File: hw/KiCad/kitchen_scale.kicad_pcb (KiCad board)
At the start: 2 copper layers, 59 x 50 mm, 11 parts, among them J1 Conn_01x08_Socket, J2 Conn_HX711, SW1 SW_Push, SW2 SW_SPST, SW3 SW_Push, SW4 SW_Push, U1 DEBO1_3_7LI_1_0A charge_contr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, U2 WeMos_D1_mini, U3 LF33_TO220

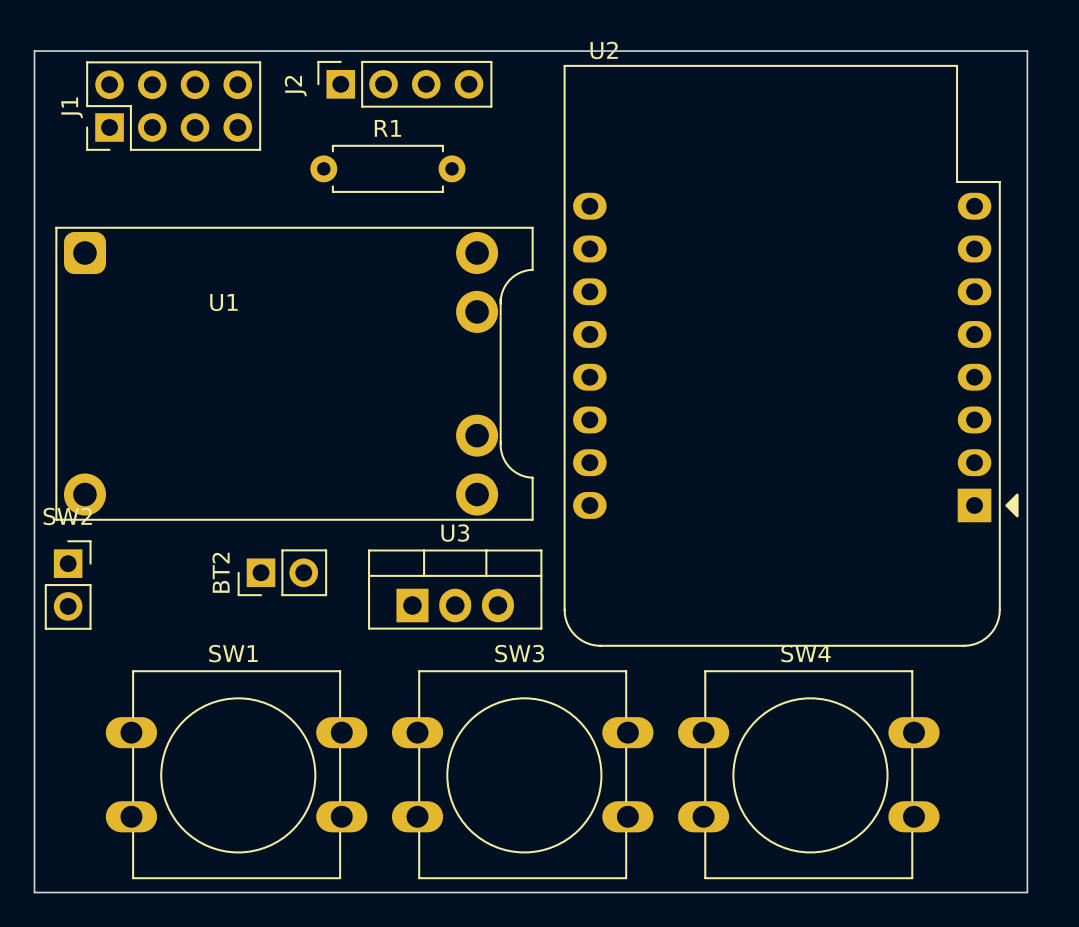
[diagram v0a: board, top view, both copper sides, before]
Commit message: Update of fine placement
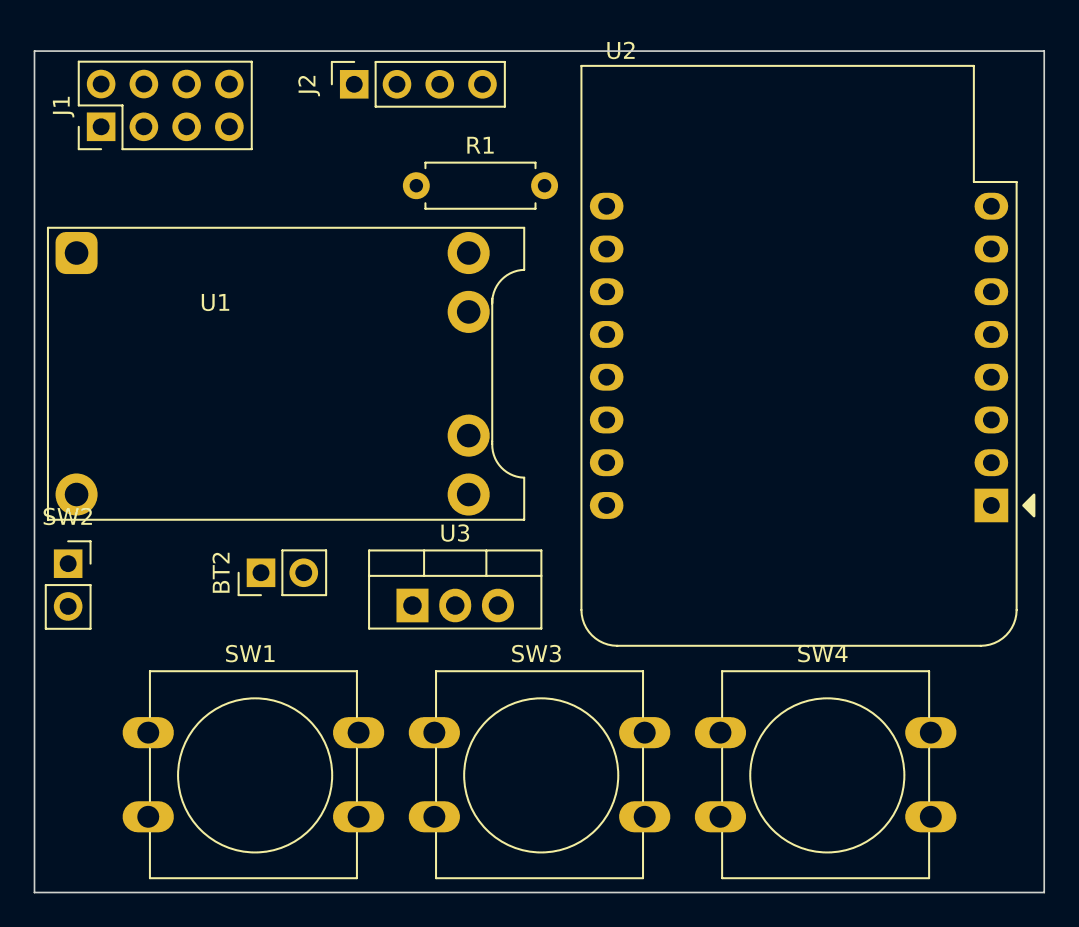
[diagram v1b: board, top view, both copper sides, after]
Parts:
- moved R1 5.59 mm to (82.7, 83.0)
- moved SW1 1.00 mm to (66.8, 115.5)
- moved SW3 1.00 mm to (83.8, 115.5)
- moved SW4 1.00 mm to (100.8, 115.5)
- moved U2 1.00 mm to (116.9, 102.0)
- moved J2 0.80 mm to (79.0, 77.0)
- moved J1 0.50 mm to (64.0, 79.5)
- moved U1 0.50 mm to (60.8, 92.5)
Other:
- board size 59 x 50 mm -> 60 x 50 mm
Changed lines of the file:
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@@
   (net 22 "unconnected-(U2-TX-Pad16)")
   (footprint "Button_Switch_THT:SW_PUSH-12mm" (layer "F.Cu")
-    (at 65.76 115.5)
+    (at 66.76 115.5)
     (descr "SW PUSH 12mm https://www.e-switch.com/system/asset/product_line/data_sheet/143/TL1100.pdf")
     (tags "tact sw push 12mm")
@@
   )
   (footprint "Connector_PinSocket_2.54mm:PinSocket_1x04_P2.54mm_Vertical" (layer "F.Cu")
-    (at 78.2 76.975 90)
+    (at 79 76.975 90)
     (descr "Through hole straight socket strip, 1x04, 2.54mm pitch, single row (from Kicad 4.0.7), script generated")
     (tags "Through hole socket strip THT 1x04 2.54mm single row")
@@
   )
   (footprint "Button_Switch_THT:SW_PUSH-12mm" (layer "F.Cu")
-    (at 82.76 115.5)
+    (at 83.76 115.5)
     (descr "SW PUSH 12mm https://www.e-switch.com/system/asset/product_line/data_sheet/143/TL1100.pdf")
     (tags "tact sw push 12mm")
@@
   )
   (footprint "Resistor_THT:R_Axial_DIN0207_L6.3mm_D2.5mm_P7.62mm_Horizontal" (layer "F.Cu")
-    (at 77.19 82)
+    (at 82.69 83)
     (descr "Resistor, Axial_DIN0207 series, Axial, Horizontal, pin pitch=7.62mm, 0.25W = 1/4W, length*diameter=6.3*2.5mm^2, http://cdn-reichelt.de/documents/datenblatt/B400/1_4W%23YAG.pdf")
     (tags "Resistor Axial_DIN0207 series Axial Horizontal pin pitch 7.62mm 0.25W = 1/4W length 6.3mm diameter 2.5mm")
@@
   )
   (footprint "Mine:DEBO1_3_7LI_1_0A_charge_controller" (layer "F.Cu")
-    (at 61.3 92.5)
+    (at 60.8 92.5)
     (descr "Texas Instruments EUS 5 Pin Double Sided Module")
     (tags "module pcb")
@@
   )
   (footprint "Module:WEMOS_D1_mini_light" (layer "F.Cu")
-    (at 115.86 102 180)
+    (at 116.86 102 180)
     (descr "16-pin module, column spacing 22.86 mm (900 mils), https://wiki.wemos.cc/products:d1:d1_mini, https://c1.staticflickr.com/1/734/31400410271_f278b087db_z.jpg")
     (tags "ESP8266 WiFi microcontroller")
@@
   )
   (footprint "Connector_PinHeader_2.54mm:PinHeader_2x04_P2.54mm_Vertical" (layer "F.Cu")
-    (at 64.46 79.54 90)
+    (at 63.96 79.5 90)
     (descr "Through hole straight pin header, 2x04, 2.54mm pitch, double rows")
     (tags "Through hole pin header THT 2x04 2.54mm double row")
@@
   )
   (footprint "Button_Switch_THT:SW_PUSH-12mm" (layer "F.Cu")
-    (at 99.76 115.5)
+    (at 100.76 115.5)
     (descr "SW PUSH 12mm https://www.e-switch.com/system/asset/product_line/data_sheet/143/TL1100.pdf")
     (tags "tact sw push 12mm")
@@
     )
   )
-  (gr_rect (start 60 75) (end 119 125)
+  (gr_rect (start 60 75) (end 120 125)
     (stroke (width 0.1) (type default)) (fill none) (layer "Edge.Cuts"))
 )
